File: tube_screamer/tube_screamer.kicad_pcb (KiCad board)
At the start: 2 copper layers, 80 x 100 mm, 68 parts, among them J1 Jack_6.35, J2 Jack_6.35, J3 Conn_01x05, J4 Conn_01x05, J5 Conn_01x05, J6 Barrel_Jack_Switch, J7 Conn_01x01_Socket, J8 Conn_01x01_Socket, P1 tube_screamer_front_panel, Q1 MMBT5551, Q2 MMBT5551, Q3 MMBT5551, SW1 pedala_switch, U1 NE5532

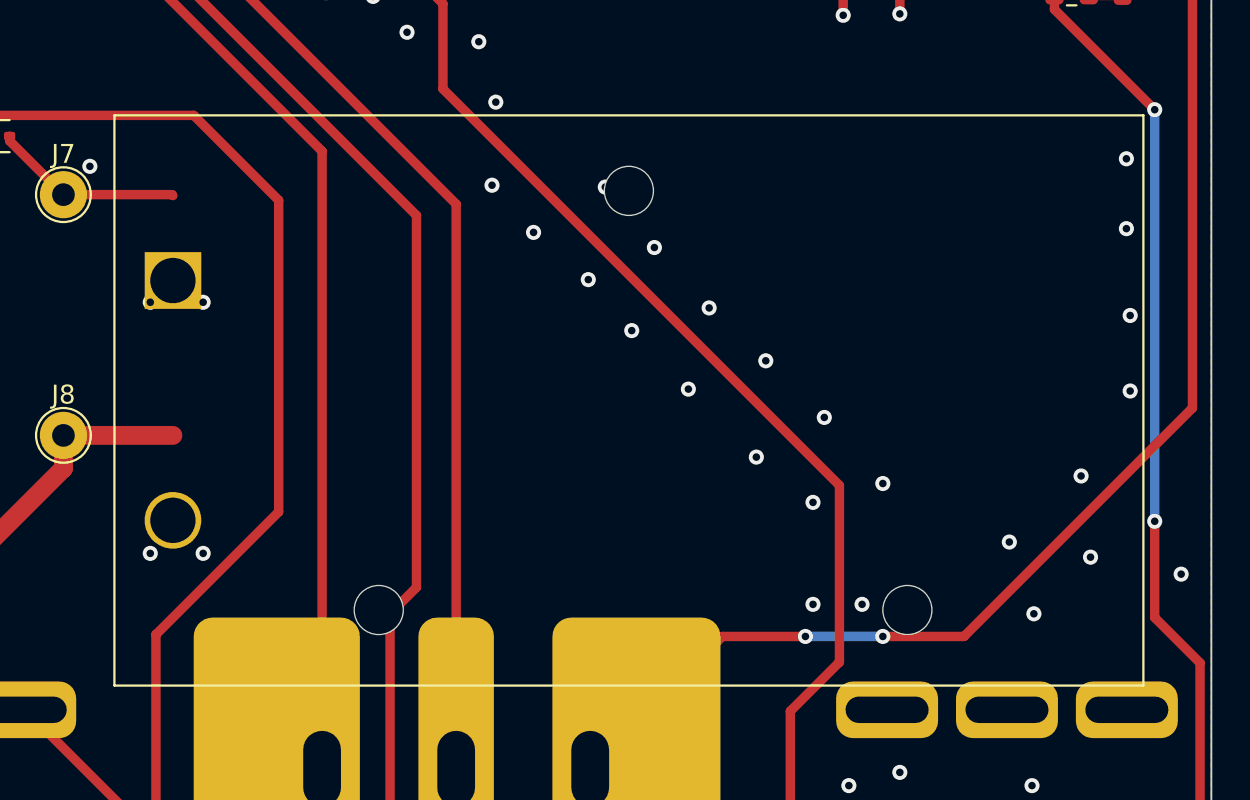
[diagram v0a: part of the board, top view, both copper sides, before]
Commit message: Update library.
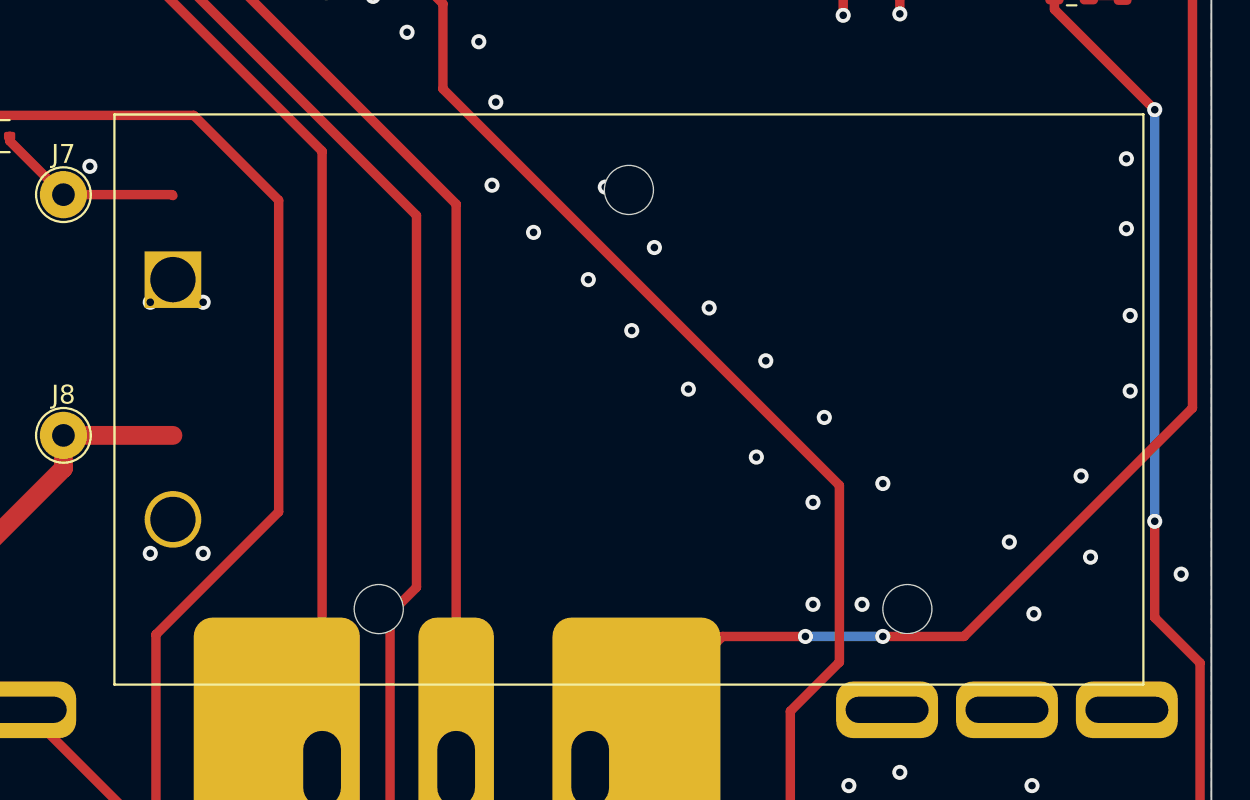
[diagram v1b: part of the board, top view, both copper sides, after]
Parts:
- moved BT1 0.05 mm to (75.0, 94.1)
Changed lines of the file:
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@@
 		(locked yes)
 		(layer "F.Cu")
-		(at 75 94.15 180)
+		(at 75 94.1 180)
 		(descr "https://eu.mouser.com/datasheet/2/209/EPD-200766-1274481.pdf")
 		(tags "9V Battery Holder")

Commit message: Updated, added 3d bodies.
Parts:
- added P2: bottom_plate, pedale:bottom_plate, F.Cu at (50.0, 50.0)
- P1: value tube_screamer_front_panel -> front_plate; footprint pedale:tube_screamer_front_plate -> pedale:front_plate
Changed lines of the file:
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@@
 		)
 		(embedded_fonts no)
-		(model "${KICAD9_3DMODEL_DIR}/Battery.3dshapes/BatteryHolder_Eagle_12BH611-GR.wrl"
+		(model "${KIPRJMOD}/../pedale.pretty/9V-battery_holder.step"
 			(offset
-				(xyz 0 0 0)
+				(xyz -25 6.5 0)
 			)
 			(scale
@@
 			)
 			(rotate
-				(xyz 0 0 0)
+				(xyz -0 -0 -0)
 			)
 		)
@@
 		(model "${KIPRJMOD}/../pedale.pretty/M3x8 Philips Screw.stp"
 			(offset
-				(xyz 0 0 -1.5)
+				(xyz 0 0 -8)
 			)
 			(scale
@@
 			)
 		)
+		(model "${KIPRJMOD}/../pedale.pretty/Abstandhalter M3 IG-AG 5mm+6mm - PA 66.stp"
+			(offset
+				(xyz 0 0 -4)
+			)
+			(scale
+				(xyz 1 1 1)
+			)
+			(rotate
+				(xyz -0 90 -0)
+			)
+		)
 	)
 	(footprint "pedale:M3_hole_with_spacer"
@@
 		(model "${KIPRJMOD}/../pedale.pretty/M3x8 Philips Screw.stp"
 			(offset
-				(xyz 0 0 -1.5)
+				(xyz 0 0 -8)
 			)
 			(scale
@@
 			)
 		)
+		(model "${KIPRJMOD}/../pedale.pretty/Abstandhalter M3 IG-AG 5mm+6mm - PA 66.stp"
+			(offset
+				(xyz 0 0 -4)
+			)
+			(scale
+				(xyz 1 1 1)
+			)
+			(rotate
+				(xyz -0 90 -0)
+			)
+		)
 	)
 	(footprint "Capacitor_SMD:C_0603_1608Metric_Pad1.08x0.95mm_HandSolder"
@@
 		)
 	)
+	(footprint "pedale:bottom_plate"
+		(layer "F.Cu")
+		(at 50 50)
+		(property "Reference" "P2"
+			(at 0 -0.5 0)
+			(unlocked yes)
+			(layer "F.SilkS")
+			(hide yes)
+			(effects
+				(font
+					(size 1 1)
+					(thickness 0.1)
+				)
+			)
+		)
+		(property "Value" "bottom_plate"
+			(at 0 1 0)
+			(unlocked yes)
+			(layer "F.Fab")
+			(effects
+				(font
+					(size 1 1)
+					(thickness 0.15)
+				)
+			)
+		)
+		(property "Datasheet" ""
+			(at 0 0 0)
+			(unlocked yes)
+			(layer "F.Fab")
+			(hide yes)
+			(effects
+				(font
+					(size 1 1)
+					(thickness 0.15)
+				)
+			)
+		)
+		(property "Description" "Potentiometer"
+			(at 0 0 0)
+			(unlocked yes)
+			(layer "F.Fab")
+			(hide yes)
+			(effects
+				(font
+					(size 1 1)
+					(thickness 0.15)
+				)
+			)
+		)
+		(property ki_fp_filters "Potentiometer*")
+		(sheetname "/")
+		(sheetfile "tube_screamer.kicad_sch")
+		(attr through_hole)
+		(fp_rect
+			(start -0.1 -0.1)
+			(end 0.1 0.1)
+			(stroke
+				(width 0.05)
+				(type default)
+			)
+			(fill no)
+			(layer "B.CrtYd")
+		)
+		(fp_text user "${REFERENCE}"
+			(at 0 2.5 0)
+			(unlocked yes)
+			(layer "F.Fab")
+			(effects
+				(font
+					(size 1 1)
+					(thickness 0.15)
+				)
+			)
+		)
+		(embedded_fonts no)
+		(model "${KIPRJMOD}/../bottom_plate.step"
+			(offset
+				(xyz 0 0 -8)
+			)
+			(scale
+				(xyz 1 1 1)
+			)
+			(rotate
+				(xyz -0 -0 -0)
+			)
+		)
+	)
 	(footprint "Resistor_SMD:R_0603_1608Metric_Pad0.98x0.95mm_HandSolder"
 		(layer "F.Cu")
@@
 		(model "${KIPRJMOD}/../pedale.pretty/M3x8 Philips Screw.stp"
 			(offset
-				(xyz 0 0 -1.5)
+				(xyz 0 0 -8)
 			)
 			(scale
@@
 			)
 		)
+		(model "${KIPRJMOD}/../pedale.pretty/Abstandhalter M3 IG-AG 5mm+6mm - PA 66.stp"
+			(offset
+				(xyz 0 0 -4)
+			)
+			(scale
+				(xyz 1 1 1)
+			)
+			(rotate
+				(xyz -0 90 -0)
+			)
+		)
 	)
 	(footprint "Capacitor_SMD:C_0603_1608Metric_Pad1.08x0.95mm_HandSolder"
@@
 		(model "${KIPRJMOD}/../pedale.pretty/M3x8 Philips Screw.stp"
 			(offset
-				(xyz 0 0 -1.5)
+				(xyz 0 0 -8)
 			)
 			(scale
@@
 			)
 		)
+		(model "${KIPRJMOD}/../pedale.pretty/Abstandhalter M3 IG-AG 5mm+6mm - PA 66.stp"
+			(offset
+				(xyz 0 0 -4)
+			)
+			(scale
+				(xyz 1 1 1)
+			)
+			(rotate
+				(xyz -0 90 -0)
+			)
+		)
 	)
 	(footprint "Resistor_SMD:R_0603_1608Metric_Pad0.98x0.95mm_HandSolder"
@@
 		)
 	)
-	(footprint "pedale:tube_screamer_front_plate"
+	(footprint "pedale:front_plate"
 		(layer "F.Cu")
 		(at 50 50)
@@
 			)
 		)
-		(property "Value" "tube_screamer_front_panel"
+		(property "Value" "front_plate"
 			(at 0 1 0)
 			(unlocked yes)
@@
 		)
 		(embedded_fonts no)
-		(model "/home/ostoja/Elektronika/pedale/tube_screamer/top_plate.step"
+		(model "${KIPRJMOD}/../top_plate.step"
 			(offset
 				(xyz 0 0 25)
@@
 		(model "${KIPRJMOD}/../pedale.pretty/M3x8 Philips Screw.stp"
 			(offset
-				(xyz 0 0 -1.5)
+				(xyz 0 0 -8)
 			)
 			(scale
@@
 			)
 		)
+		(model "${KIPRJMOD}/../pedale.pretty/Abstandhalter M3 IG-AG 5mm+6mm - PA 66.stp"
+			(offset
+				(xyz 0 0 -4)
+			)
+			(scale
+				(xyz 1 1 1)
+			)
+			(rotate
+				(xyz -0 90 -0)
+			)
+		)
